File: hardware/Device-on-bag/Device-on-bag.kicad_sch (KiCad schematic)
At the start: 2 parts, among them U1 SparkFun_SEN-14480_H3LIS331DL, U2 ESP32-DEVKIT-V1

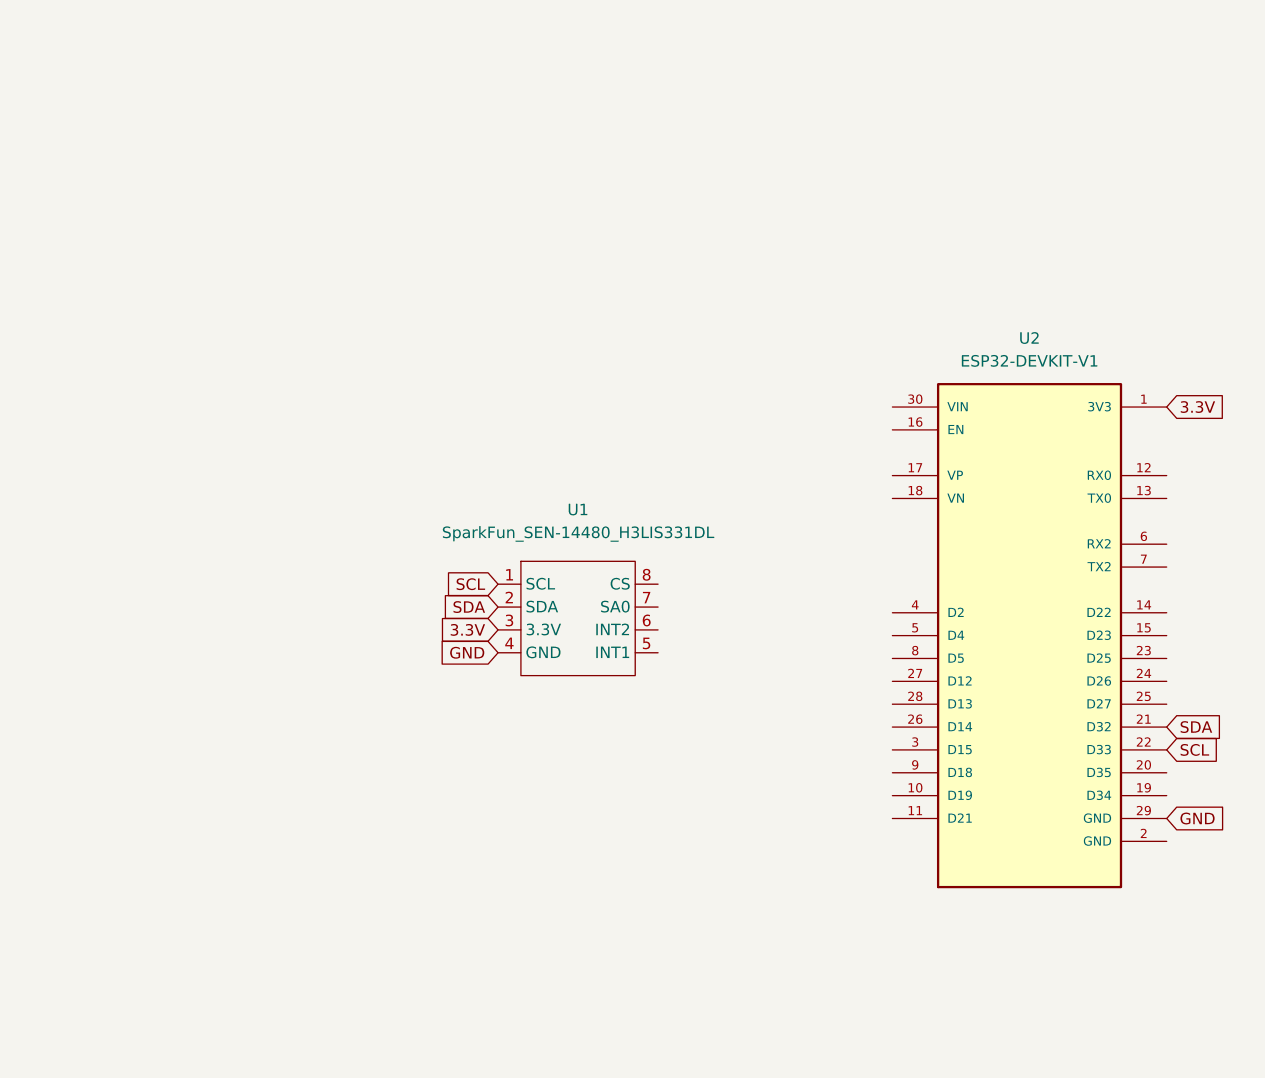
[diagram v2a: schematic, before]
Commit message: update
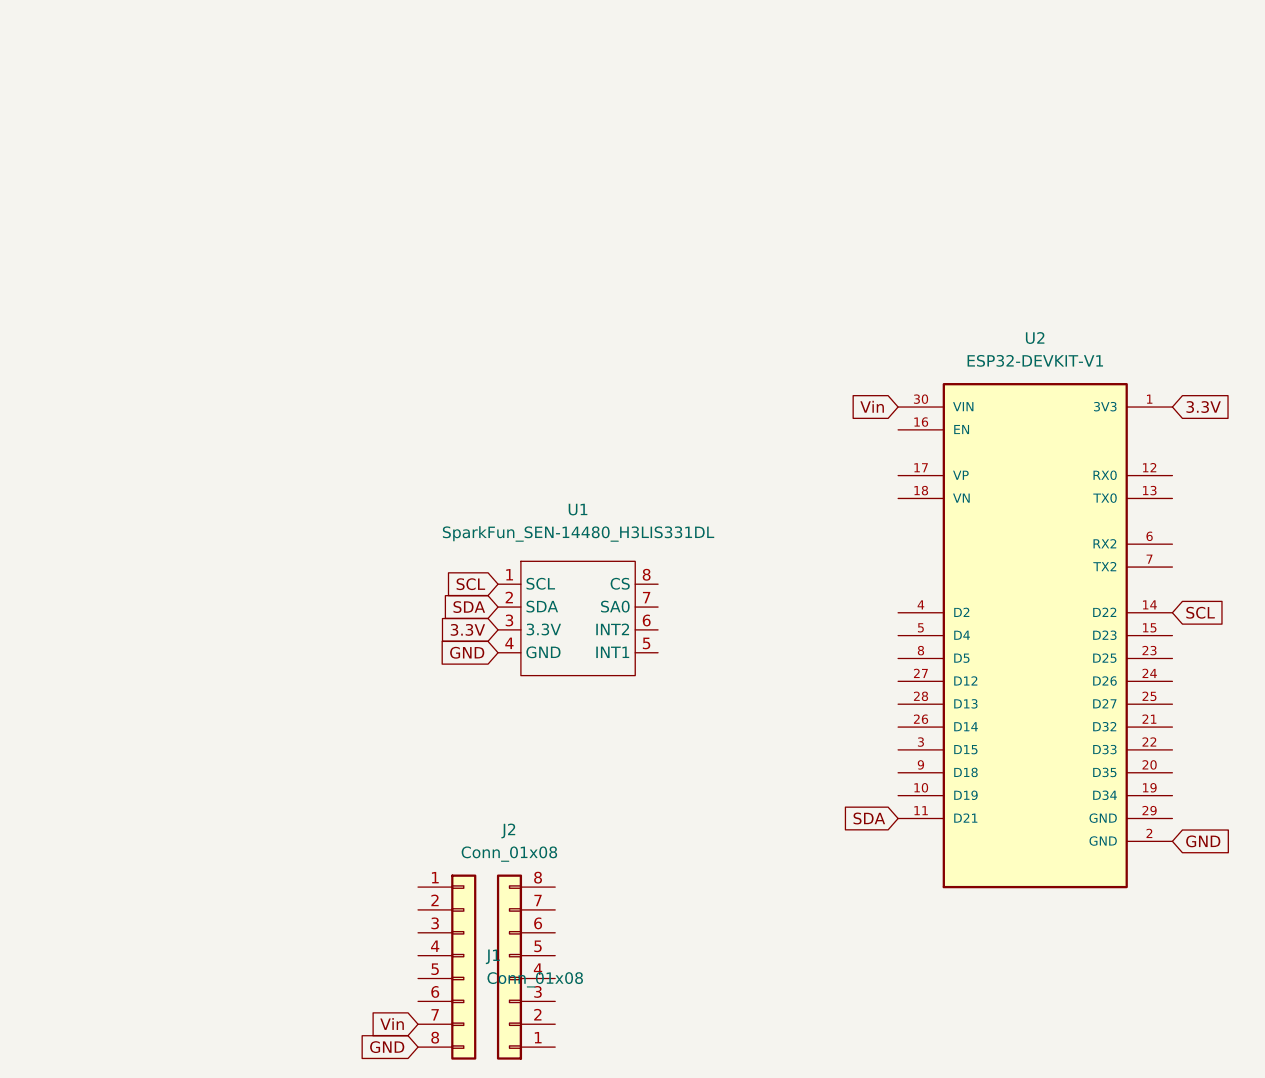
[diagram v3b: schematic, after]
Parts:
- added J1, J2: Conn_01x08, Connector_PinSocket_2.54mm:PinSocket_1x08_P2.54mm_Vertical, symbol Connector_Generic:Conn_01x08
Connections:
- net GND: now also U2.2 (GND), J1.8 (Pin_8); no longer U2.29 (GND)
- net SCL: now also U2.14 (D22); no longer U2.22 (D33)
- net SDA: now also U2.11 (D21); no longer U2.21 (D32)
- net Vin: now reaches U2.30 (VIN)
- net Vin: now also J1.7 (Pin_7)
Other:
- moved on the sheet: U2
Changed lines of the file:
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@@
     )
   )
-  (global_label "SCL" (shape input) (at 192.405 111.76 0) (fields_autoplaced)
-    (effects (font (size 1.27 1.27)) (justify left))
-    (property "Intersheet References" "${INTERSHEET_REFS}" (id 0) (at 198.3257 111.6806 0)
-      (effects (font (size 1.27 1.27)) (justify left) hide)
+  (global_label "Vin" (shape input) (at 109.22 142.24 180) (fields_autoplaced)
+    (effects (font (size 1.27 1.27)) (justify right))
+    (property "Intersheet References" "${INTERSHEET_REFS}" (id 0) (at 103.9645 142.1606 0)
+      (effects (font (size 1.27 1.27)) (justify right) hide)
+    )
+  )
+  (global_label "Vin" (shape input) (at 162.56 73.66 180) (fields_autoplaced)
+    (effects (font (size 1.27 1.27)) (justify right))
+    (property "Intersheet References" "${INTERSHEET_REFS}" (id 0) (at 157.3045 73.5806 0)
+      (effects (font (size 1.27 1.27)) (justify right) hide)
     )
   )
@@
     )
   )
-  (global_label "GND" (shape input) (at 192.405 119.38 0) (fields_autoplaced)
+  (global_label "GND" (shape input) (at 193.04 121.92 0) (fields_autoplaced)
     (effects (font (size 1.27 1.27)) (justify left))
-    (property "Intersheet References" "${INTERSHEET_REFS}" (id 0) (at 198.6886 119.4594 0)
+    (property "Intersheet References" "${INTERSHEET_REFS}" (id 0) (at 199.3236 121.9994 0)
       (effects (font (size 1.27 1.27)) (justify left) hide)
     )
   )
-  (global_label "3.3V" (shape input) (at 192.405 73.66 0) (fields_autoplaced)
+  (global_label "GND" (shape input) (at 109.22 144.78 180) (fields_autoplaced)
+    (effects (font (size 1.27 1.27)) (justify right))
+    (property "Intersheet References" "${INTERSHEET_REFS}" (id 0) (at 102.9364 144.7006 0)
+      (effects (font (size 1.27 1.27)) (justify right) hide)
+    )
+  )
+  (global_label "3.3V" (shape input) (at 193.04 73.66 0) (fields_autoplaced)
     (effects (font (size 1.27 1.27)) (justify left))
-    (property "Intersheet References" "${INTERSHEET_REFS}" (id 0) (at 198.9305 73.5806 0)
+    (property "Intersheet References" "${INTERSHEET_REFS}" (id 0) (at 199.5655 73.5806 0)
       (effects (font (size 1.27 1.27)) (justify left) hide)
     )
   )
-  (global_label "SDA" (shape input) (at 192.405 109.22 0) (fields_autoplaced)
-    (effects (font (size 1.27 1.27)) (justify left))
-    (property "Intersheet References" "${INTERSHEET_REFS}" (id 0) (at 198.3862 109.1406 0)
-      (effects (font (size 1.27 1.27)) (justify left) hide)
+  (global_label "SDA" (shape input) (at 162.56 119.38 180) (fields_autoplaced)
+    (effects (font (size 1.27 1.27)) (justify right))
+    (property "Intersheet References" "${INTERSHEET_REFS}" (id 0) (at 156.5788 119.4594 0)
+      (effects (font (size 1.27 1.27)) (justify right) hide)
     )
   )
@@
     )
   )
+  (global_label "SCL" (shape input) (at 193.04 96.52 0) (fields_autoplaced)
+    (effects (font (size 1.27 1.27)) (justify left))
+    (property "Intersheet References" "${INTERSHEET_REFS}" (id 0) (at 198.9607 96.4406 0)
+      (effects (font (size 1.27 1.27)) (justify left) hide)
+    )
+  )
   (global_label "SDA" (shape input) (at 118.11 95.885 180) (fields_autoplaced)
     (effects (font (size 1.27 1.27)) (justify right))
@@
       (effects (font (size 1.27 1.27)) (justify right) hide)
     )
+  )
+  (symbol (lib_id "Connector_Generic:Conn_01x08") (at 119.38 137.16 180) (unit 1)
+    (in_bom yes) (on_board yes) (fields_autoplaced)
+    (property "Reference" "J2" (id 0) (at 119.38 120.65 0))
+    (property "Value" "Conn_01x08" (id 1) (at 119.38 123.19 0))
+    (property "Footprint" "Connector_PinSocket_2.54mm:PinSocket_1x08_P2.54mm_Vertical" (id 2) (at 119.38 137.16 0)
+      (effects (font (size 1.27 1.27)) hide)
+    )
+    (property "Datasheet" "~" (id 3) (at 119.38 137.16 0)
+      (effects (font (size 1.27 1.27)) hide)
+    )
+    (pin "1")
+    (pin "2")
+    (pin "3")
+    (pin "4")
+    (pin "5")
+    (pin "6")
+    (pin "7")
+    (pin "8")
+  )
+  (symbol (lib_id "Connector_Generic:Conn_01x08") (at 114.3 134.62 0) (unit 1)
+    (in_bom yes) (on_board yes) (fields_autoplaced)
+    (property "Reference" "J1" (id 0) (at 116.84 134.6199 0)
+      (effects (font (size 1.27 1.27)) (justify left))
+    )
+    (property "Value" "Conn_01x08" (id 1) (at 116.84 137.1599 0)
+      (effects (font (size 1.27 1.27)) (justify left))
+    )
+    (property "Footprint" "Connector_PinSocket_2.54mm:PinSocket_1x08_P2.54mm_Vertical" (id 2) (at 114.3 134.62 0)
+      (effects (font (size 1.27 1.27)) hide)
+    )
+    (property "Datasheet" "~" (id 3) (at 114.3 134.62 0)
+      (effects (font (size 1.27 1.27)) hide)
+    )
+    (pin "1")
+    (pin "2")
+    (pin "3")
+    (pin "4")
+    (pin "5")
+    (pin "6")
+    (pin "7")
+    (pin "8")
   )
   (symbol (lib_id "H3LIS331DL:SparkFun_SEN-14480_H3LIS331DL") (at 127 97.155 0) (unit 1)
@@
     (pin "8")
   )
-  (symbol (lib_id "ESP32-DEVKIT-V1:ESP32-DEVKIT-V1") (at 177.165 99.06 0) (unit 1)
+  (symbol (lib_id "ESP32-DEVKIT-V1:ESP32-DEVKIT-V1") (at 177.8 99.06 0) (unit 1)
     (in_bom yes) (on_board yes) (fields_autoplaced)
-    (property "Reference" "U2" (id 0) (at 177.165 66.04 0))
-    (property "Value" "ESP32-DEVKIT-V1" (id 1) (at 177.165 68.58 0))
-    (property "Footprint" "MODULE_ESP32_DEVKIT_V1" (id 2) (at 165.735 62.23 0)
+    (property "Reference" "U2" (id 0) (at 177.8 66.04 0))
+    (property "Value" "ESP32-DEVKIT-V1" (id 1) (at 177.8 68.58 0))
+    (property "Footprint" "MODULE_ESP32_DEVKIT_V1" (id 2) (at 166.37 62.23 0)
       (effects (font (size 1.27 1.27)) (justify left bottom) hide)
     )
-    (property "Datasheet" "" (id 3) (at 177.165 99.06 0)
+    (property "Datasheet" "" (id 3) (at 177.8 99.06 0)
       (effects (font (size 1.27 1.27)) (justify left bottom) hide)
     )
-    (property "STANDARD" "Manufacturer Recommendations" (id 4) (at 163.195 64.77 0)
+    (property "STANDARD" "Manufacturer Recommendations" (id 4) (at 163.83 64.77 0)
       (effects (font (size 1.27 1.27)) (justify left bottom) hide)
     )
-    (property "PARTREV" "N/A" (id 5) (at 184.785 67.31 0)
+    (property "PARTREV" "N/A" (id 5) (at 185.42 67.31 0)
       (effects (font (size 1.27 1.27)) (justify left bottom) hide)
     )
-    (property "MANUFACTURER" "DOIT" (id 6) (at 191.135 62.23 0)
+    (property "MANUFACTURER" "DOIT" (id 6) (at 191.77 62.23 0)
       (effects (font (size 1.27 1.27)) (justify left bottom) hide)
     )
-    (property "MAXIMUM_PACKAGE_HEIGHT" "6.8 mm" (id 7) (at 183.515 69.85 0)
+    (property "MAXIMUM_PACKAGE_HEIGHT" "6.8 mm" (id 7) (at 184.15 69.85 0)
       (effects (font (size 1.27 1.27)) (justify left bottom) hide)
     )
@@
   )
   (symbol_instances
+    (path "/8e909e36-2ea6-4b97-ad8a-8a0879639875"
+      (reference "J1") (unit 1) (value "Conn_01x08") (footprint "Connector_PinSocket_2.54mm:PinSocket_1x08_P2.54mm_Vertical")
+    )
+    (path "/173b3a26-c401-4096-bbdf-e51853bf08d7"
+      (reference "J2") (unit 1) (value "Conn_01x08") (footprint "Connector_PinSocket_2.54mm:PinSocket_1x08_P2.54mm_Vertical")
+    )
     (path "/bdadbb5c-7221-4007-9a12-2ce8f2e20049"
       (reference "U1") (unit 1) (value "SparkFun_SEN-14480_H3LIS331DL") (footprint "SparkFun_Tri_Axis_Accel_Breakout-H3LIS331DL:SparkFun_Tri_Axis_Accel_Breakout-H3LIS331DL")
